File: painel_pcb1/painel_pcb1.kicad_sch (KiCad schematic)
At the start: 58 parts, among them J1 Conn_02x16_Counter_Clockwise, J2 Conn_02x02_Counter_Clockwise, J3 Conn_02x06_Counter_Clockwise, J4 Conn_02x08_Counter_Clockwise, J5 Conn_02x03_Counter_Clockwise, J6 Conn_02x08_Counter_Clockwise, U1 MAX7219, U2 MAX7219, U3 74LS595, U4 74LS595, U5 Pico

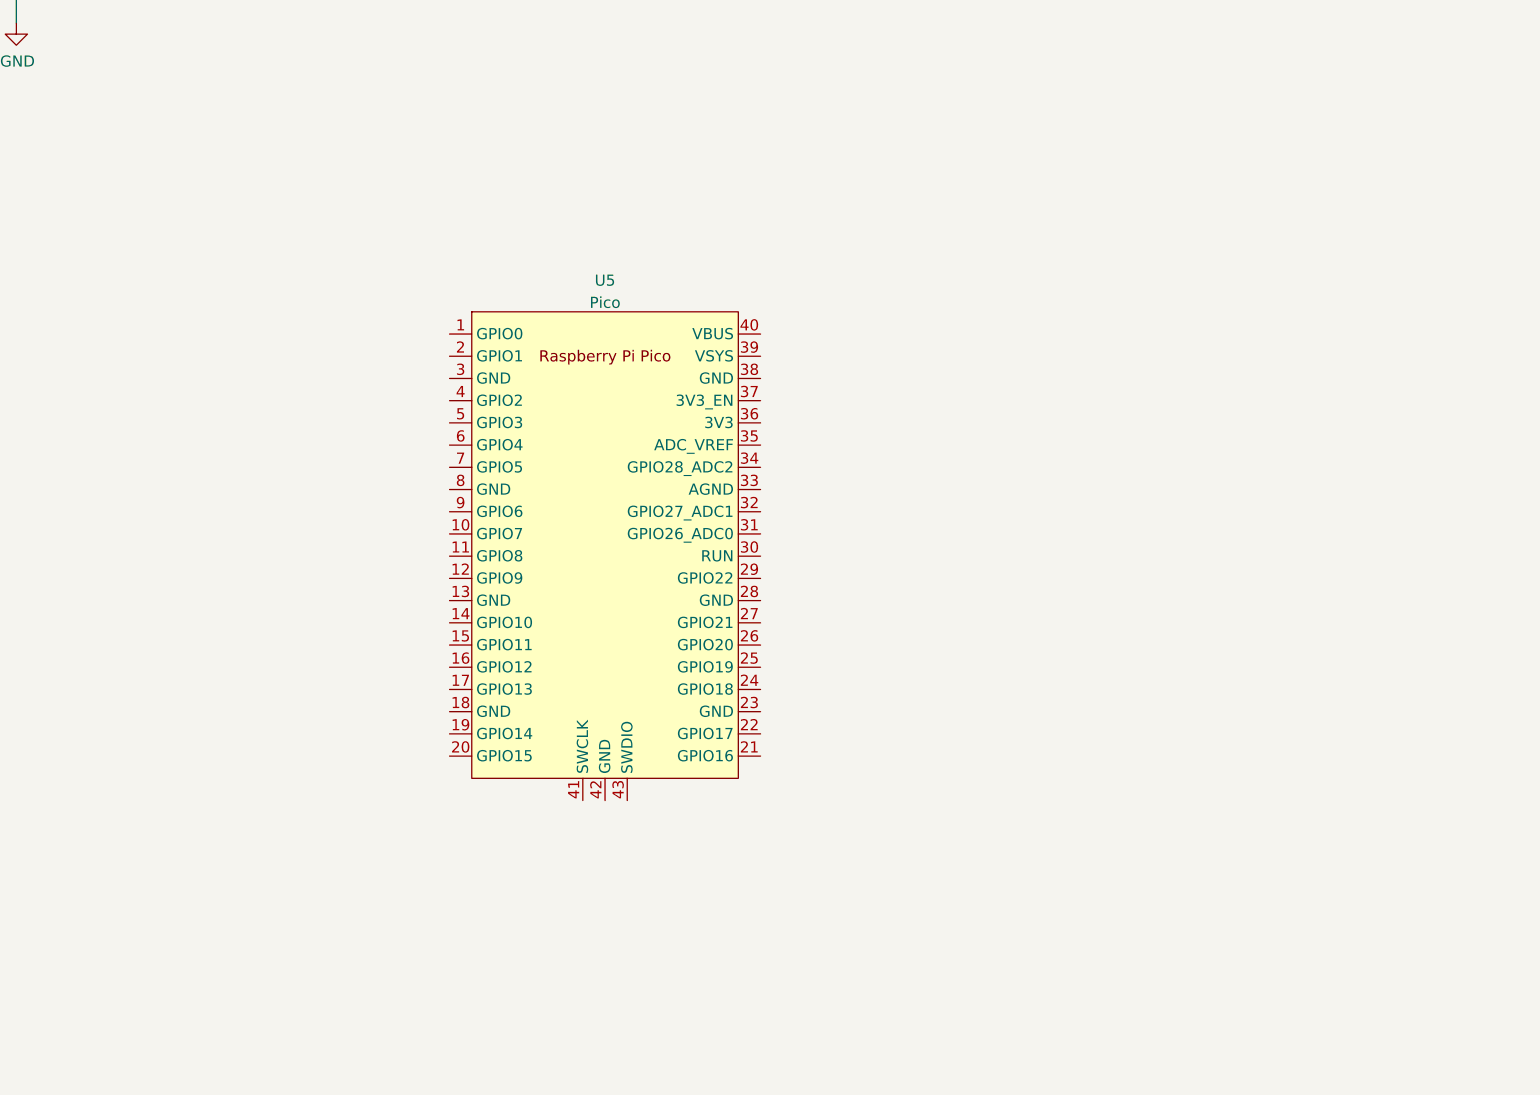
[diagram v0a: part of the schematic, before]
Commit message: wip
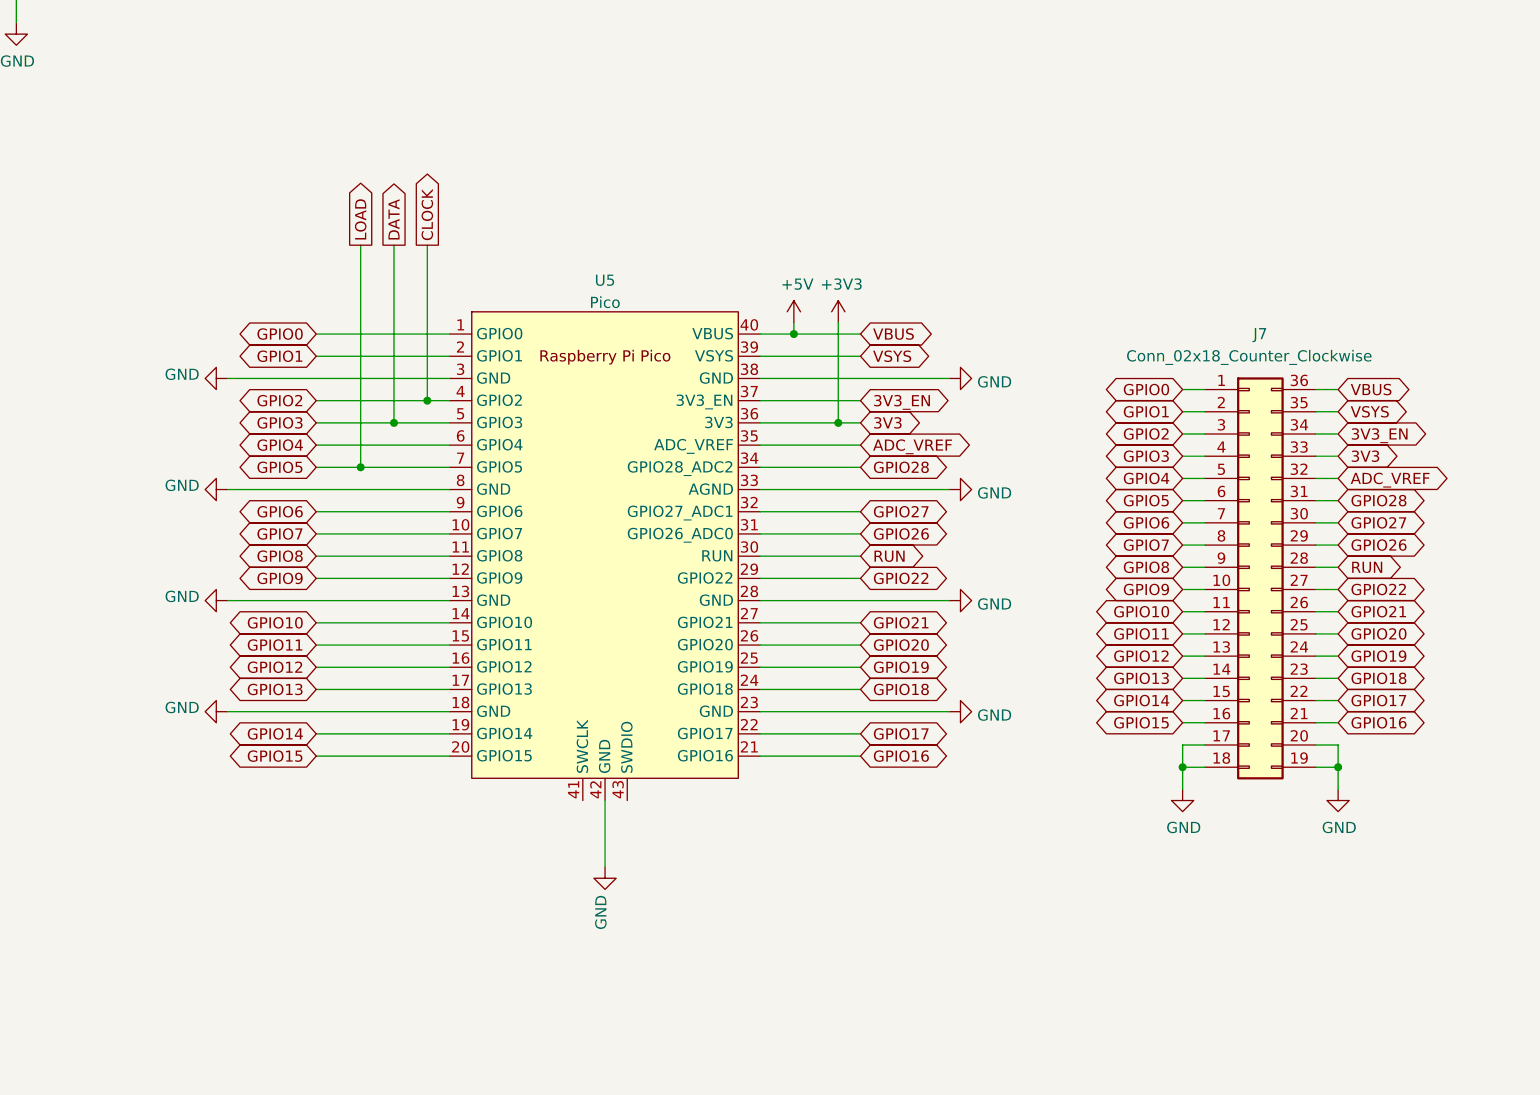
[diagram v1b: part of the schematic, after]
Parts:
- added J7: Conn_02x18_Counter_Clockwise, Connector_PinHeader_2.54mm:PinHeader_2x18_P2.54mm_Vertical, symbol Connector_Generic:Conn_02x18_Counter_Clockwise
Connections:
- net +3V3: now also U5.36 (3V3), J7.33 (Pin_33)
- net +5V: now also U5.40 (VBUS), J7.36 (Pin_36)
- net CLOCK: now also U5.4 (GPIO2), J7.3 (Pin_3)
- net D2: now also U5.5 (GPIO3), J7.4 (Pin_4)
- net D3: now also U5.7 (GPIO5), J7.6 (Pin_6)
- net GND: now also U5.13 (GND), U5.18 (GND), U5.23 (GND), U5.28 (GND), U5.3 (GND), U5.33 (AGND), U5.38 (GND), U5.42 (GND), U5.8 (GND), J7.17 (Pin_17), J7.18 (Pin_18), J7.19 (Pin_19), J7.20 (Pin_20)
- net GPIO0: now reaches U5.1 (GPIO0)
- net GPIO0: now also J7.1 (Pin_1)
- net GPIO7: now reaches U5.10 (GPIO7)
- net GPIO7: now also J7.8 (Pin_8)
- net GPIO8: now reaches U5.11 (GPIO8)
- net GPIO8: now also J7.9 (Pin_9)
- net GPIO9: now reaches U5.12 (GPIO9)
- net GPIO9: now also J7.10 (Pin_10)
- net GPIO10: now reaches U5.14 (GPIO10)
- net GPIO10: now also J7.11 (Pin_11)
- net GPIO11: now reaches U5.15 (GPIO11)
- net GPIO11: now also J7.12 (Pin_12)
- net GPIO12: now reaches U5.16 (GPIO12)
- net GPIO12: now also J7.13 (Pin_13)
- net GPIO13: now reaches U5.17 (GPIO13)
- net GPIO13: now also J7.14 (Pin_14)
- net GPIO14: now reaches U5.19 (GPIO14)
- net GPIO14: now also J7.15 (Pin_15)
- net GPIO1: now reaches U5.2 (GPIO1)
- net GPIO1: now also J7.2 (Pin_2)
- net GPIO15: now reaches U5.20 (GPIO15)
- net GPIO15: now also J7.16 (Pin_16)
- net GPIO16: now reaches U5.21 (GPIO16)
- net GPIO16: now also J7.21 (Pin_21)
- net GPIO17: now reaches U5.22 (GPIO17)
- net GPIO17: now also J7.22 (Pin_22)
- net GPIO18: now reaches U5.24 (GPIO18)
- net GPIO18: now also J7.23 (Pin_23)
- net GPIO19: now reaches U5.25 (GPIO19)
- net GPIO19: now also J7.24 (Pin_24)
- net GPIO20: now reaches U5.26 (GPIO20)
- net GPIO20: now also J7.25 (Pin_25)
- net GPIO21: now reaches U5.27 (GPIO21)
- net GPIO21: now also J7.26 (Pin_26)
- net GPIO22: now reaches U5.29 (GPIO22)
- net GPIO22: now also J7.27 (Pin_27)
- net RUN: now reaches U5.30 (RUN)
- net RUN: now also J7.28 (Pin_28)
- net GPIO26: now reaches U5.31 (GPIO26_ADC0)
- net GPIO26: now also J7.29 (Pin_29)
- net GPIO27: now reaches U5.32 (GPIO27_ADC1)
- net GPIO27: now also J7.30 (Pin_30)
- net GPIO28: now reaches U5.34 (GPIO28_ADC2)
- net GPIO28: now also J7.31 (Pin_31)
- net ADC_VREF: now reaches U5.35 (ADC_VREF)
- net ADC_VREF: now also J7.32 (Pin_32)
- net 3V3_EN: now reaches U5.37 (3V3_EN)
- net 3V3_EN: now also J7.34 (Pin_34)
- net VSYS: now reaches U5.39 (VSYS)
- net VSYS: now also J7.35 (Pin_35)
- net GPIO4: now reaches U5.6 (GPIO4)
- net GPIO4: now also J7.5 (Pin_5)
- net GPIO6: now reaches U5.9 (GPIO6)
- net GPIO6: now also J7.7 (Pin_7)
